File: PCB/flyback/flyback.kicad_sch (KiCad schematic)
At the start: 7 parts, among them T1 Transformer_1P_1S

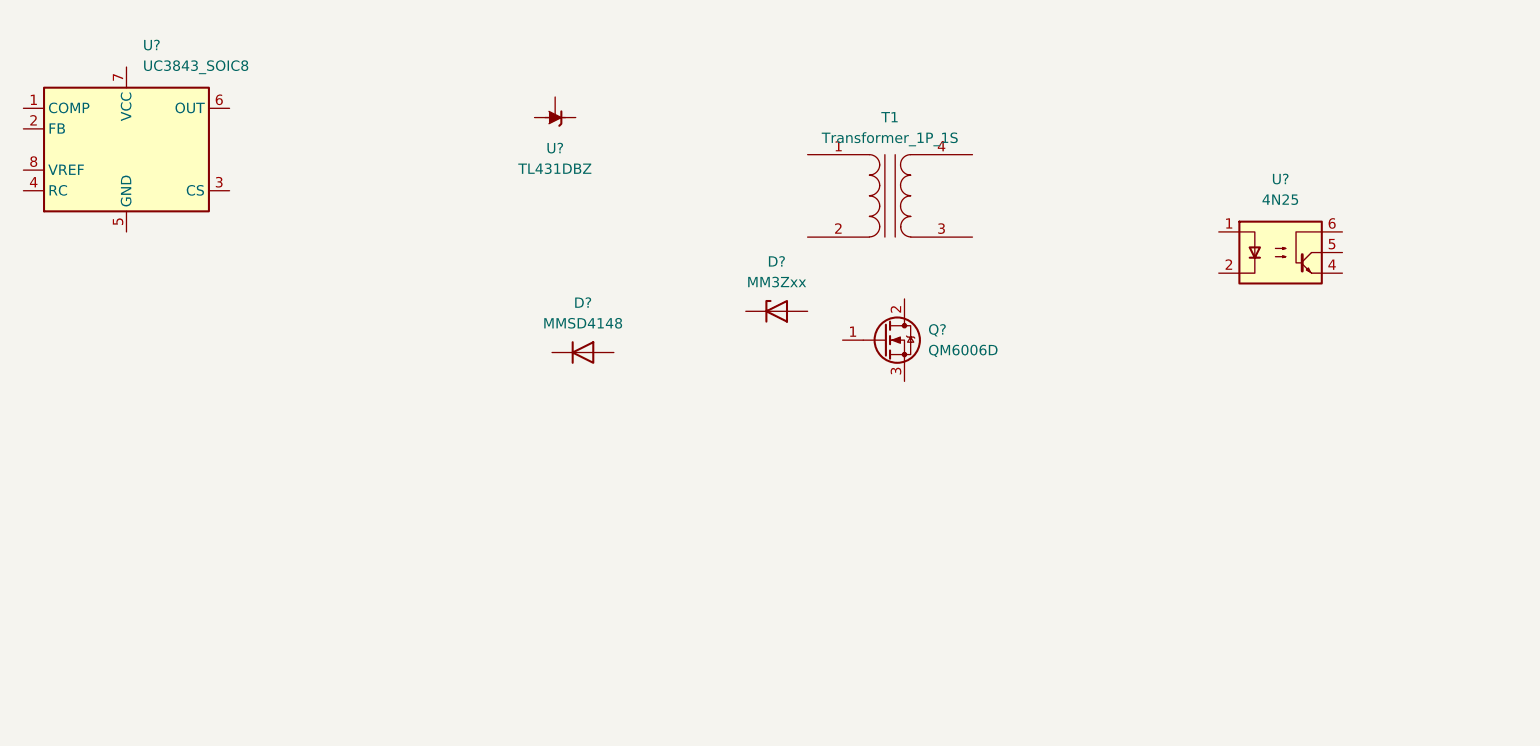
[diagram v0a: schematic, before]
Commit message: Schematic Update
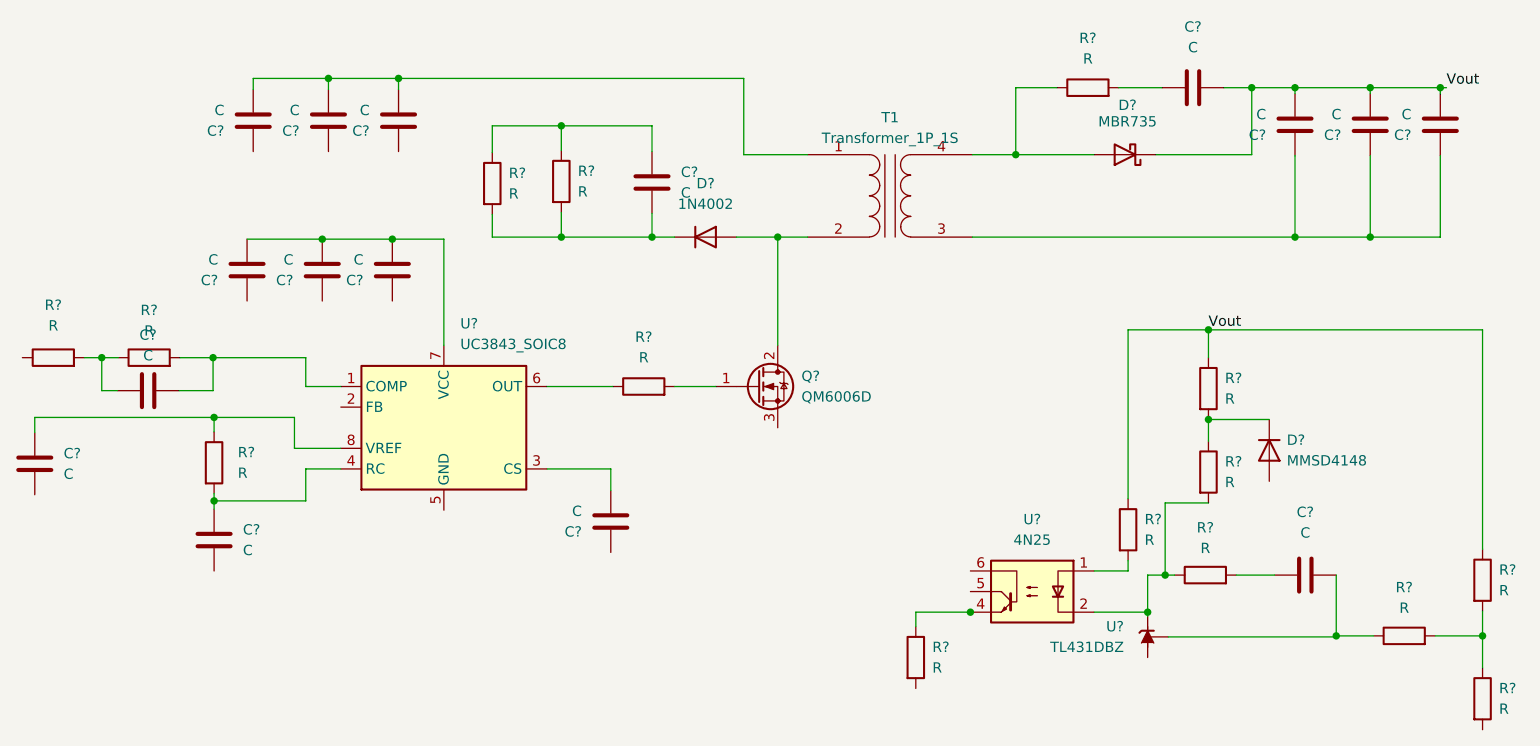
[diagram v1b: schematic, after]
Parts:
- removed D?: MM3Zxx, Diode_SMD:D_SOD-323F, symbol Diode:MM3Zxx
- added C? (x16): C, symbol Device:C
- added D?: 1N4002, Diode_THT:D_DO-41_SOD81_P10.16mm_Horizontal, symbol Diode:1N4002
- added D?: MBR735, Package_TO_SOT_THT:TO-220-2_Vertical, symbol Diode:MBR735
- added R? (x15): R, symbol Device:R
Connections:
- net at Q?.1 (G): now also R?.2
- net at Q?.2 (D): now also T1.2 (AB), D?.2 (A)
- net at U?.1: now also R?.2
- net at U?.2: now also U?.1 (K), R?.1, R?.2
- net at U?.4: now also R?.1
- net at U?.1 (COMP): now also C?.2, R?.2
- net at U?.3 (CS): now also C?.2
- net at U?.4 (RC): now also C?.1, R?.2
- net at U?.6 (OUT): now also R?.1
- net at U?.7 (VCC): now also C?.2, C?.2, C?.2
- net at U?.8 (VREF): now also C?.1, R?.1
- net at T1.1 (AA): now also C?.2, C?.2, C?.2
- net at T1.3 (SA): now also C?.1, C?.1, C?.1
- net at T1.4 (SB): now also D?.2 (A), R?.1
- net at U?.2 (REF): now also C?.2, R?.1
- net at D?.1 (K): now also R?.1, R?.2
- new net: C?.1, R?.2 (x2)
- new net: C?.1, R?.1, R?.2
- new net: R?.1, R?.2, R?.2
- new net: C?.1, R?.1, R?.1
- new net: C?.2, D?.1 (K), R?.2, R?.2
- new net Vout: C?.2, C?.2, C?.2, C?.2, D?.1 (K), R?.1, R?.1, R?.1
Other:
- moved on the sheet: D?, Q?, U?
